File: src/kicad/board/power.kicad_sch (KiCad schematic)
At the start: 21 parts, among them Q1 DMG2305UX, U2 BQ25172, U3 TLV61070A, U4 XC6206P332MR

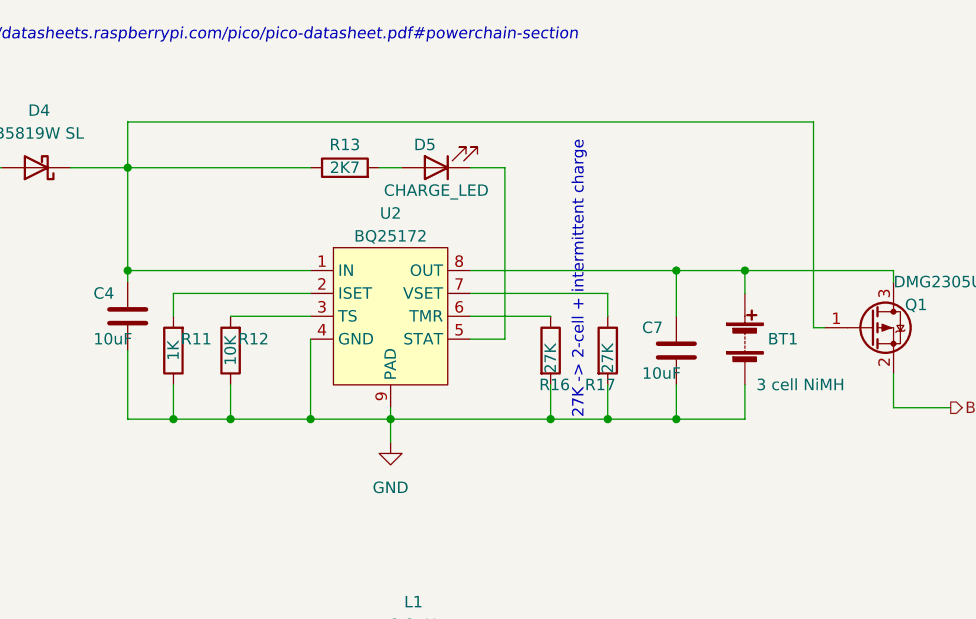
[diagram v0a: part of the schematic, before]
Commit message: updated with new pcb
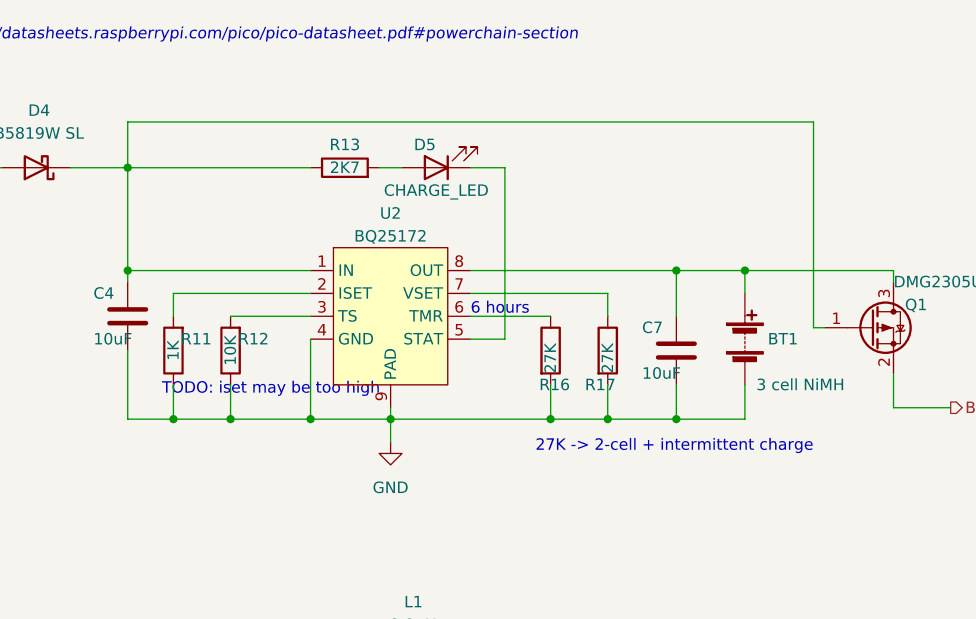
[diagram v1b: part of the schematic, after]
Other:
- note added: "6 hours"
- note added: "TODO: iset may be too high"
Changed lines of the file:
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@@
     (stroke (width 0) (type default) (color 0 0 0 0))
+  )
+  (text "TODO: iset may be too high\n" (at 111.76 71.12 0)
+    (effects (font (size 1.27 1.27)) (justify left bottom))
   )
   (text "TODO: reduce coil whine" (at 125.73 134.62 0)
     (effects (font (size 1.27 1.27)) (justify left bottom))
   )
-  (text "27K -> 2-cell + intermittent charge\n" (at 158.75 73.66 90)
-    (effects (font (size 1.27 1.27)) (justify left bottom))
+  (text "27K -> 2-cell + intermittent charge\n" (at 184.15 77.47 180)
+    (effects (font (size 1.27 1.27)) (justify right bottom))
   )
   (text "https://datasheets.raspberrypi.com/pico/pico-datasheet.pdf#powerchain-section"
@@
     (effects (font (size 1.27 1.27) italic) (justify left bottom))
   )
+  (text "6 hours\n" (at 146.05 62.23 0)
+    (effects (font (size 1.27 1.27)) (justify left bottom))
+  )
   (hierarchical_label "3.3V_OUT" (shape output) (at 204.47 132.08 0)
